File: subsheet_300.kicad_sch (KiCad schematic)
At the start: 37 parts, among them Q11 2N3904, Q6 2N3904, Q7 2N3906, Q8 2N3904, Q9 2N3906, U41 74LS74 DUAL FLIP-FLOPS, Y2 see table, Y3 see table

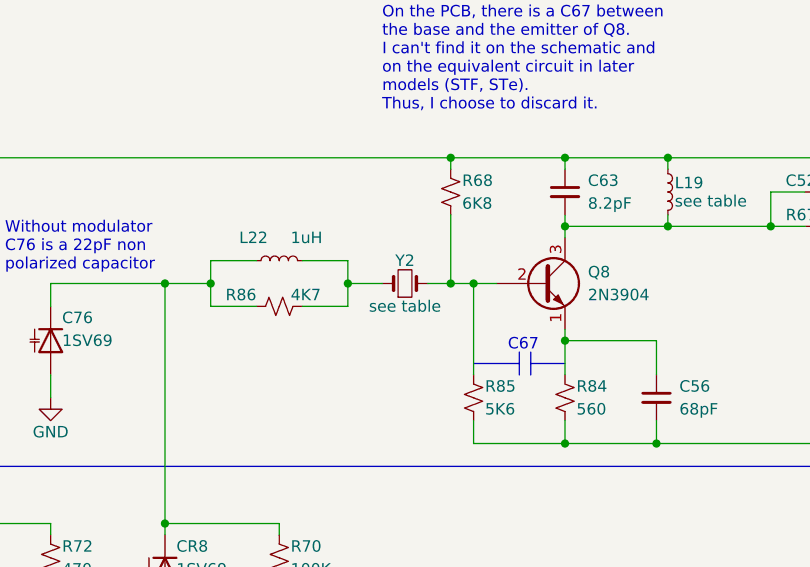
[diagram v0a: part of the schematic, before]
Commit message: pcb session : acsi port, floppy disc drive port, parts of 32Mhz clock and modulator clock -- 2023-08-16T08:43+02:00
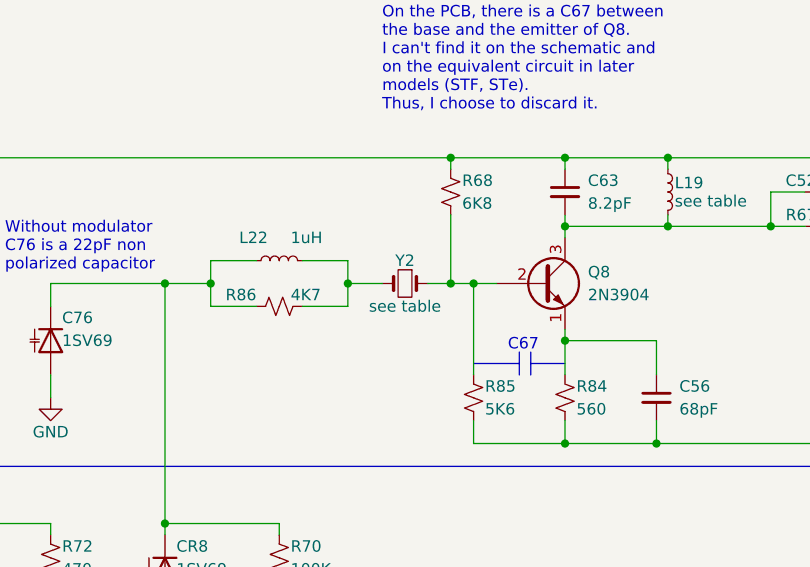
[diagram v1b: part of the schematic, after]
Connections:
- net at Q8.2 (B), R68.1, R85.2: now also Y2.1; no longer Y2.2
- net at L22.2, R86.2: now also Y2.2; no longer Y2.1
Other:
- moved on the sheet: Y2
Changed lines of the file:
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@@
     (pin "2")
   )
-  (symbol (lib_id "Device:Crystal_Small") (at 99.06 48.26 0) (unit 1)
+  (symbol (lib_id "Device:Crystal_Small") (at 99.06 48.26 180) (unit 1)
     (in_bom yes) (on_board yes)
     (property "Reference" "Y2" (id 0) (at 99.06 45.72 0))

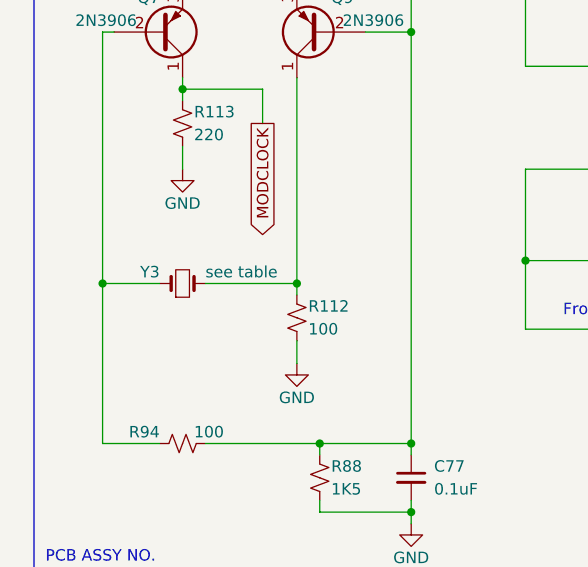
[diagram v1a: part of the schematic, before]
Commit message: pcb session : done positionning, but traces will not match -- 2023-08-16T16:57+02:00
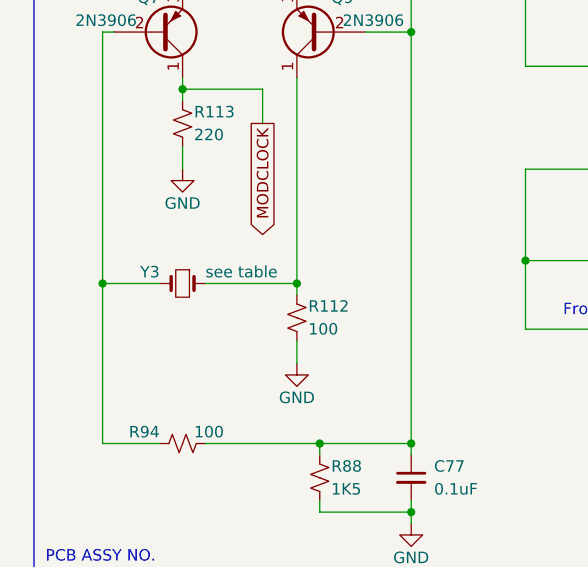
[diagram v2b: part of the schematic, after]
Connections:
- net at Q9.1 (C), R112.2: now also Y3.1; no longer Y3.2
- net at Q7.2 (B), R94.1: now also Y3.2; no longer Y3.1
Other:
- moved on the sheet: Y3
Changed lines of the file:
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@@
     (pin "2")
   )
-  (symbol (lib_id "Device:Crystal_Small") (at 34.29 116.84 0) (unit 1)
+  (symbol (lib_id "Device:Crystal_Small") (at 34.29 116.84 180) (unit 1)
     (in_bom yes) (on_board yes)
     (property "Reference" "Y3" (id 0) (at 31.75 115.57 0)
+      (effects (font (size 1.27 1.27)) (justify left))
+    )
+    (property "Value" "see table" (id 1) (at 36.83 115.57 0)
       (effects (font (size 1.27 1.27)) (justify right))
     )
-    (property "Value" "see table" (id 1) (at 36.83 115.57 0)
-      (effects (font (size 1.27 1.27)) (justify left))
-    )
     (property "Footprint" "Crystal:Crystal_HC50_Horizontal" (id 2) (at 34.29 116.84 0)
